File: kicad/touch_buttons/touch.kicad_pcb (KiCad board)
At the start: 2 copper layers, 15.7 x 15.7 mm, 3 parts, among them J1 CONN_01X03

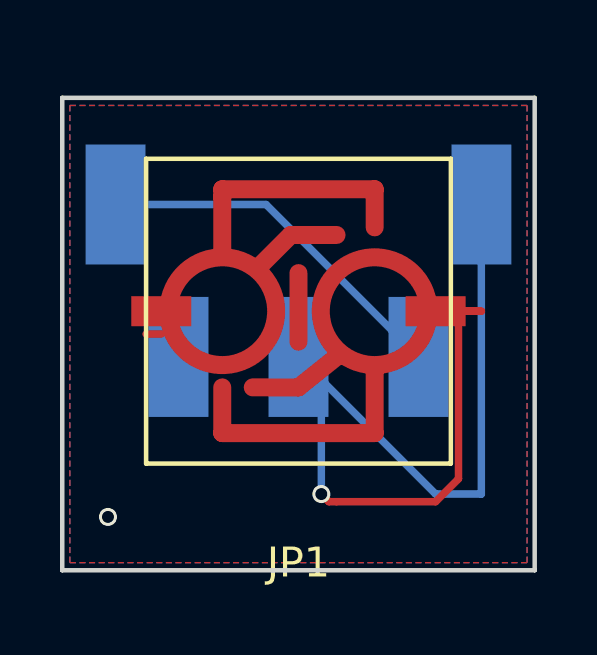
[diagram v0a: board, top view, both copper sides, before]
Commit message: update
- drawing buttons
- still to finish
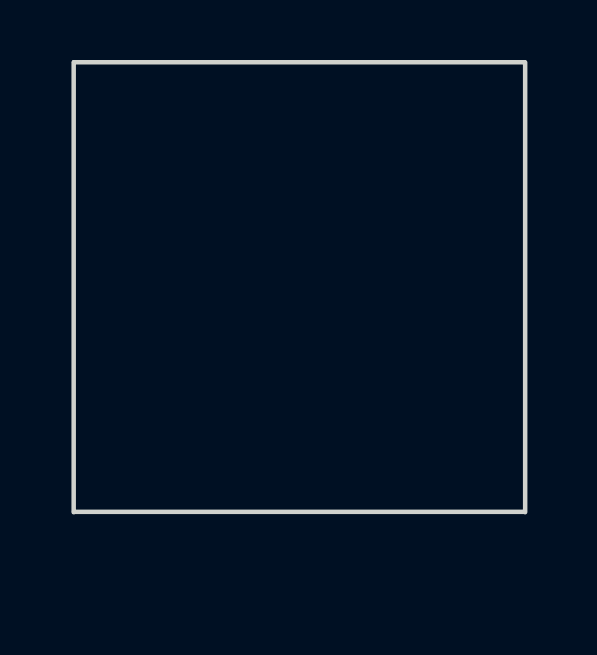
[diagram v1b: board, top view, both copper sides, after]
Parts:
- removed 2M1: R, Touch_conn:res
- removed J1: CONN_01X03, Touch_conn:touch_conn
- removed JP1: touch, Touch_conn:touch
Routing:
- net Net-(2M1-Pad2): track 36.9 -> 0.00 mm, vias 1 -> 0
- net Net-(2M1-Pad1): track 12.2 -> 0.00 mm
- net (no net): track 0.51 -> 0.00 mm, vias 1 -> 0
- removed copper zone on B.Cu, net GND
- removed copper zone on F.Cu, net GND
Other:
- board size 15.7 x 15.7 mm -> 15 x 15 mm
